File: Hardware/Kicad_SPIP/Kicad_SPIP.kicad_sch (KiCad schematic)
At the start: 29 parts, among them J1 Conn_01x03, J2 Conn_01x02, J3 Conn_01x04, J4 Conn_01x06, J5 Conn_01x06, J6 Conn_01x06, SW1 SW_Push, SW2 SW_Push, SW3 SW_Push, U1 STM32G431CBUx, U2 STM32G431CBU6, U3 DRV8411APWPR

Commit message: pcb 1.2
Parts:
- removed SW2: SW_Push, symbol Switch:SW_Push
- removed U1: STM32G431CBUx, Package_DFN_QFN:QFN-48-1EP_7x7mm_P0.5mm_EP5.6x5.6mm, symbol MCU_ST_STM32G4:STM32G431CBUx
- removed U3: DRV8411APWPR, DRV8411APWPR:IC_DRV8411APWPR, symbol DRV8411A:DRV8411APWPR
- added C10, C14, C15, C16, C8: 1u, Capacitor_SMD:C_0603_1608Metric, symbol Device:C_Small
- added C11: 10u, Capacitor_SMD:CP_Elec_4x5.4, symbol Device:C_Polarized_Small
- added C13, C9: 10n, Capacitor_SMD:C_0402_1005Metric, symbol Device:C_Small
- added C17: 10n, LED_SMD:LED_0603_1608Metric, symbol Device:C_Small
- added C7: 22u, Capacitor_SMD:C_0805_2012Metric, symbol Device:C_Small
- added D1, D2: LED, LED_SMD:LED_0603_1608Metric, symbol Device:LED
- added H1, H2, H3, H4, H5, H6, H7, H8: MountingHole_Pad, MountingHole:MountingHole_3.2mm_M3_Pad_Via, symbol Mechanical:MountingHole_Pad
- added J2: Conn_ST_STDC14, Connector_PinHeader_1.27mm:PinHeader_2x07_P1.27mm_Vertical_SMD, symbol Connector:Conn_ST_STDC14
- added R12, R14, R15, R16, R2, R8, R9: 10k, Resistor_SMD:R_0402_1005Metric, symbol Device:R_Small
- added R3: 4k3, Resistor_SMD:R_0402_1005Metric, symbol Device:R_Small
- added R4: 1k6, Resistor_SMD:R_0402_1005Metric, symbol Device:R_Small
- added SW1, SW4: SW_Push, Button_Switch_SMD:SW_SPST_B3U-3000P, symbol Switch:SW_Push
- added unit 2 of U1
- added U2: AZ1117CH-3.3TRG1, Package_TO_SOT_SMD:SOT-223-3_TabPin2, symbol Regulator_Linear:AZ1117-3.3
- added U3: DRV8411APWPR, DRV8411APWPR:IC_DRV8411APWPR, symbol DRV8411APWPR:DRV8411APWPR
- C1: value 1µF -> 10u
- C12: renamed from C7; value 100nF -> 100n
- C2, C4, C5: value 100nF -> 100n
- C3: value 100nF -> 10u; footprint Capacitor_SMD:C_0402_1005Metric -> Capacitor_SMD:C_0603_1608Metric
- C6: value 1µF -> 100n; footprint Capacitor_SMD:C_0603_1608Metric -> Capacitor_SMD:C_0402_1005Metric
- D3: renamed from D1; footprint (none) -> LED_SMD:LED_0603_1608Metric; MPN (none) -> 150060BS55040
- D4: renamed from D2; footprint (none) -> LED_SMD:LED_0603_1608Metric; MPN (none) -> 150060GS55040
- D5: renamed from D3; footprint (none) -> LED_SMD:LED_0603_1608Metric; MPN (none) -> 150060RS55040
- J3: renamed from J1; footprint Connector_JST:JST_XH_B3B-XH-A_1x03_P2.50mm_Vertical -> Connector_JST:JST_PH_B3B-PH-K_1x03_P2.00mm_Vertical
- J4: renamed from J3; footprint Connector_JST:JST_XH_B4B-XH-A_1x04_P2.50mm_Vertical -> Connector_JST:JST_PH_B3B-PH-K_1x03_P2.00mm_Vertical
- J5: renamed from J4; footprint Connector_JST:JST_XH_B6B-XH-A_1x06_P2.50mm_Vertical -> Connector_JST:JST_PH_B3B-PH-K_1x03_P2.00mm_Vertical
- J6: renamed from J5; footprint Connector_JST:JST_XH_B6B-XH-A_1x06_P2.50mm_Vertical -> Connector_JST:JST_PH_B6B-PH-K_1x06_P2.00mm_Vertical
- J7: renamed from J6; footprint Connector_JST:JST_XH_B6B-XH-A_1x06_P2.50mm_Vertical -> Connector_JST:JST_PH_B6B-PH-K_1x06_P2.00mm_Vertical
- R1: value 330 Ohm -> 330; footprint Resistor_SMD:R_0805_2012Metric -> Resistor_SMD:R_0402_1005Metric
- R10: renamed from R3; value 82.5kOhm -> 82k5; footprint Resistor_SMD:R_0805_2012Metric -> Resistor_SMD:R_0402_1005Metric
- R11: renamed from R4; value 82kOhm -> 82k5; footprint Resistor_SMD:R_0805_2012Metric -> Resistor_SMD:R_0402_1005Metric
- R13: renamed from R2; value 1kOhm -> 1k
- R5: value 1k -> 680; footprint (none) -> Resistor_SMD:R_0402_1005Metric
- R6: footprint (none) -> Resistor_SMD:R_0402_1005Metric
- R7: value 1k -> 1k6; footprint (none) -> Resistor_SMD:R_0402_1005Metric
- SW2: renamed from SW1; footprint (none) -> Button_Switch_SMD:SW_SPST_B3U-3000P
- SW3: footprint (none) -> Button_Switch_SMD:SW_SPST_B3U-3000P
- U1: renamed from U2; footprint UFQFPN-48_7X7X0P55MM -> STM32G431CBU6:UFQFPN-48_7X7X0P55MM
- renumbered J2 to J1
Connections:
- net +3.3VA is gone; now on net +3.3V: C1.1, C2.1
- net +7.5V is gone; now on net +6V: J3.2 (Pin_2)
- net +3.3V: now also C6.1, C10.1, C14.1, C15.2, C16.2, C7.1, J2.3 (VCC), R14.1, R16.1, R4.2, R9.1, U1.1 (VBAT), U1.20 (VREF+), U1.21 (VDDA), U1.23 (VDD), U1.35 (VDD), U1.48 (VDD), U2.2 (VO), U3.1 (VREF); no longer C3.1
- net +6V: now also C12.1, C3.1, J1.2 (Pin_2), C11.1, C8.2, R3.2, U2.3 (VI), U3.12 (VM); no longer J1.1 (Pin_1)
- net AIN1: now also U3.16 (AIN1)
- net AIN2: now also U3.15 (AIN2)
- net AOUT1: now also U3.2 (AOUT1)
- net AOUT2: now also U3.4 (AOUT2)
- net BIN1: now also U3.9 (BIN1)
- net BIN2: now also U3.10 (BIN2)
- net BOUT1: now also U3.7 (BOUT1)
- net BOUT2: now also U3.5 (BOUT2)
- net Button1: now also C9.2, R8.1; no longer SW3.2
- net Button2: now also C13.2, R12.1
- net Button3: now also C17.2, R15.1; no longer SW2.2
- net FAULT: now also U3.8 (~{FAULT})
- net GND: now also C1.2, C12.2, C2.2, C3.2, C4.2, C5.2, C6.2, D3.1 (K), D4.1 (K), D5.1 (K), J1.1 (Pin_1), C10.2, C11.2, C13.1, C14.2, C15.1, C16.1, C17.1, C7.2, C8.1, C9.1, D1.1 (K), D2.1 (K), H1.1, H2.1, H3.1, H4.1, H5.1, H6.1, H7.1, H8.1, J2.11 (GNDDetect), J2.5 (GND), J2.7 (GND), R2.2, SW1.1, SW4.1, U1.49 (EPAD), U2.1 (GND), U3.13 (GND), U3.17 (EXP), U3.3 (PGNDA), U3.6 (PGNDB); no longer J1.2 (Pin_2), R5.1, R6.2, R7.2
- net at R11.1: now also U3.14 (AIPROPI)
- net STLINK_TX: now reaches U1.10 (PA2-UART_STLINK_TX)
- net STLINK_TX: now also J2.14 (VCP_TX)
- net STLINK_RX: now reaches U1.11 (PA3-UART_STLINK_RX)
- net STLINK_RX: now also J2.13 (VCP_RX)
- net JTMS/SWDIO: now reaches U1.36 (PA13-SYS_JTMS-SWDIO)
- net JTMS/SWDIO: now also J2.4 (JTMS/SWDIO)
- net JCLK/SWCLK: now reaches U1.37 (PA14-SYS_JTCK-SWCLK)
- net JCLK/SWCLK: now also J2.6 (JCLK/SWCLK)
- net at U1.46 (PB8-BOOT0): now also R2.1
- net NRST: now reaches U1.7 (PG10-NRST)
- net NRST: now also J2.12 (~{RST}), SW1.2
- net at R10.1: now also U3.11 (BIPROPI)
- removed net +8V: C12.1, C6.1
- net LED1 renamed LEDB
- net LEDB: now also R5.1; no longer D3.1 (K)
- net LED2 renamed LEDG
- net LEDG: now also R6.2; no longer D4.1 (K)
- net LED3 renamed LEDR
- net LEDR: now also R7.2; no longer D5.1 (K)
- new net: R15.2, R16.2, SW4.2
- new net: R12.2, R14.2, SW3.2
- new net: R8.2, R9.2, SW2.2
- new net: D1.2 (A), R3.1
- new net: D2.2 (A), R4.1
- no-connect marks 44 -> 17
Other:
- note added: "1.7V @ 1mA"
- note added: "2.3V @ 1mA"
- note added: "2.6V @ 1mA"
- note added: "Motor specification Vnom = 6V 300rpm max Istall = 200mA InoLoad = 45mA"
- note added: "MountingHole_Pad"
- note added: "Programmateur"
- moved on the sheet: C12, D3, D4, D5, J1, J3, J4, J5, J6, J7, R1, R10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

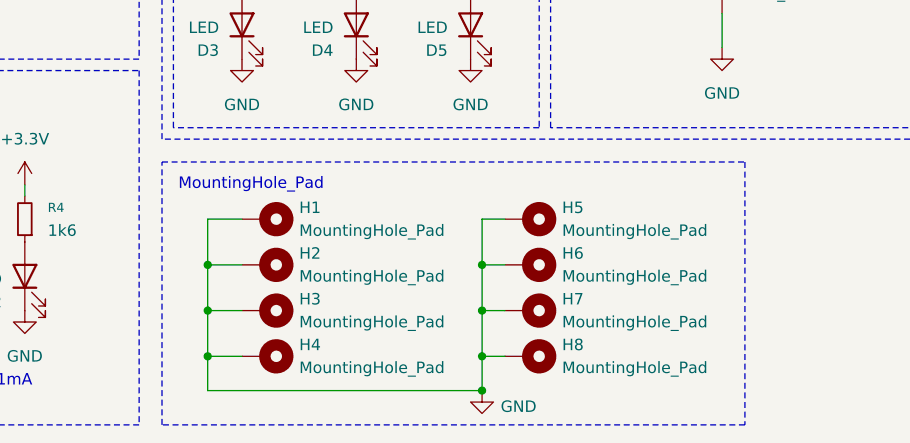
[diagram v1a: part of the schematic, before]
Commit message: pcb rootage
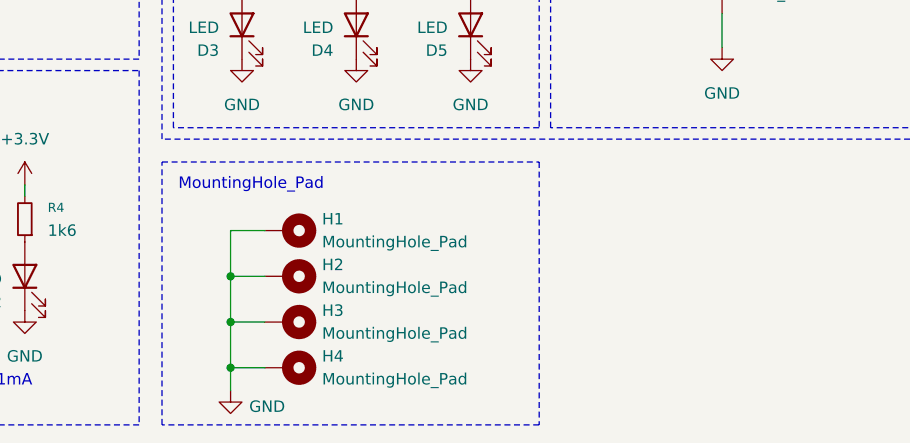
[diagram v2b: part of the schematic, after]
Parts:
- removed H5, H6, H7, H8: MountingHole_Pad, MountingHole:MountingHole_3.2mm_M3_Pad_Via, symbol Mechanical:MountingHole_Pad
- C17: footprint LED_SMD:LED_0603_1608Metric -> Capacitor_SMD:C_0402_1005Metric
- J4: footprint Connector_JST:JST_PH_B3B-PH-K_1x03_P2.00mm_Vertical -> Connector_JST:JST_PH_B4B-PH-K_1x04_P2.00mm_Vertical
- J5: footprint Connector_JST:JST_PH_B3B-PH-K_1x03_P2.00mm_Vertical -> Connector_JST:JST_PH_B6B-PH-K_1x06_P2.00mm_Vertical
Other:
- moved on the sheet: H1, H2, H3, H4
